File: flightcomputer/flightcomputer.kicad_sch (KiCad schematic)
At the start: 65 parts, among them J1 Conn_Coaxial, J10 Conn_01x03, J11 Conn_01x03, J12 282837-2, J13 282837-2, J2 Conn_Coaxial, J3 Conn_Coaxial, J4 Conn_Coaxial, J5 Conn_01x24, J6 Conn_01x24, J7 Conn_01x01, J8 Conn_01x01, J9 Conn_01x02, M1 Motor_Servo, M2 Motor_Servo, Q1 MMBT3904, Q2 MMBT3904, Q3 SI4925DDY-T1-GE3, U1 MAX-M10S, U2 LIS2MDLTR, U3 BMI088, U4 MS5607-02BA, U5 MIC29302AWD-TR, U6 RFM95W-915S2, U7 Teensy4.1, U8 LD1117S50TR_SOT223

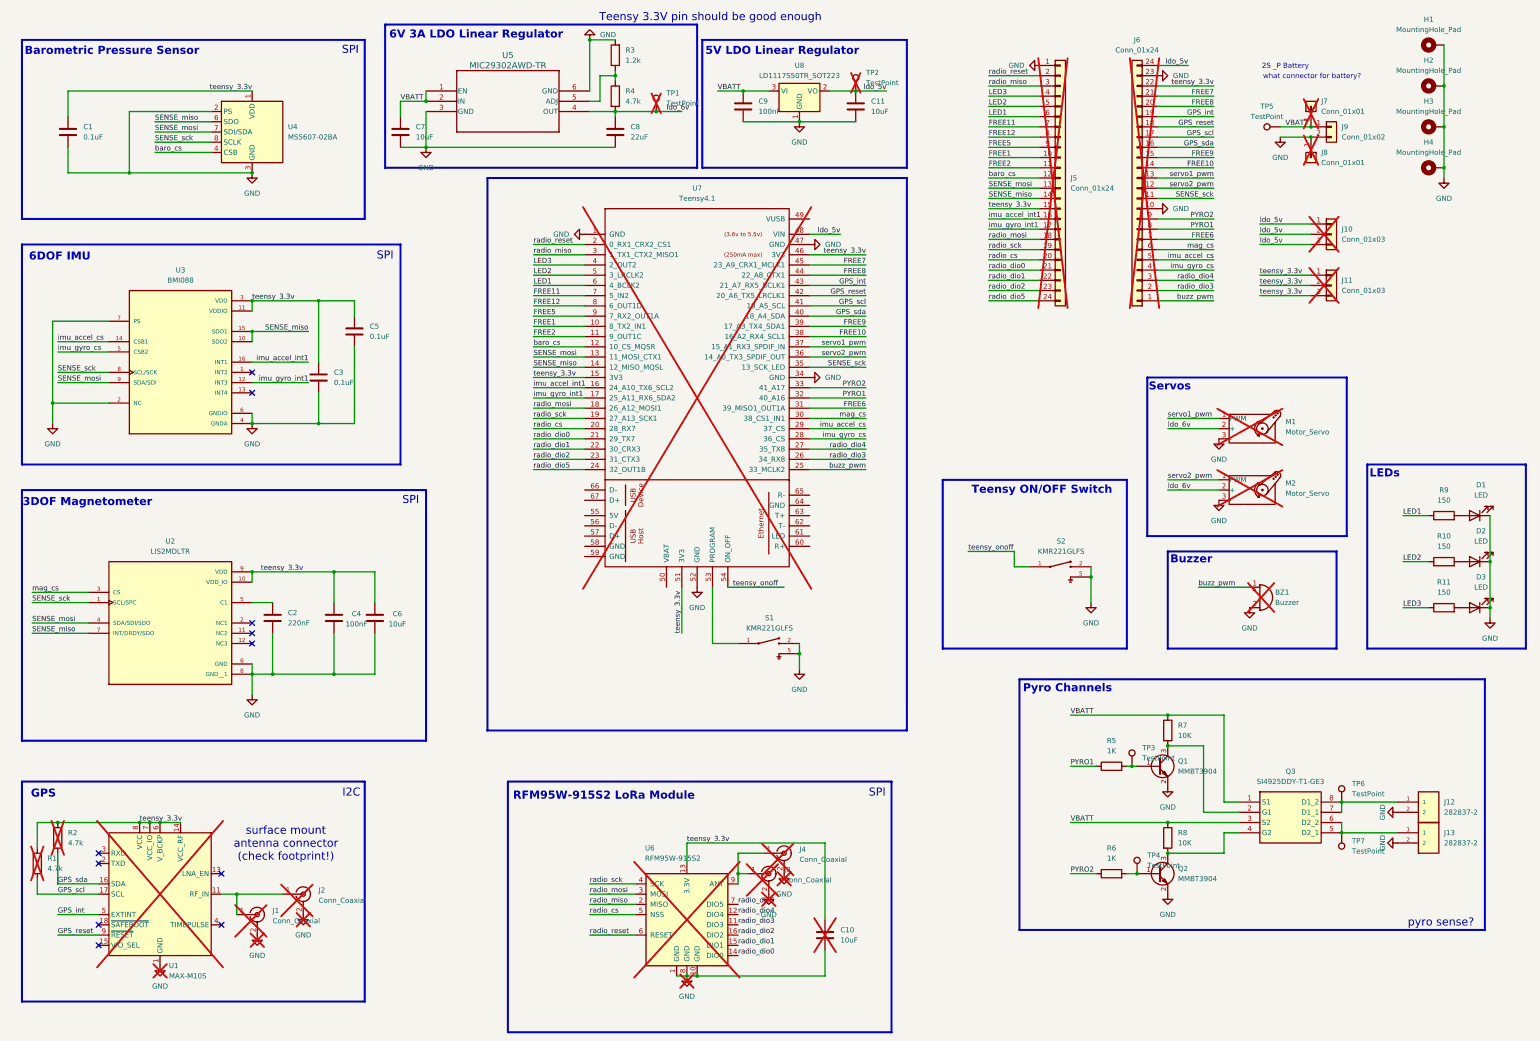
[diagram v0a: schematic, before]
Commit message: all boards
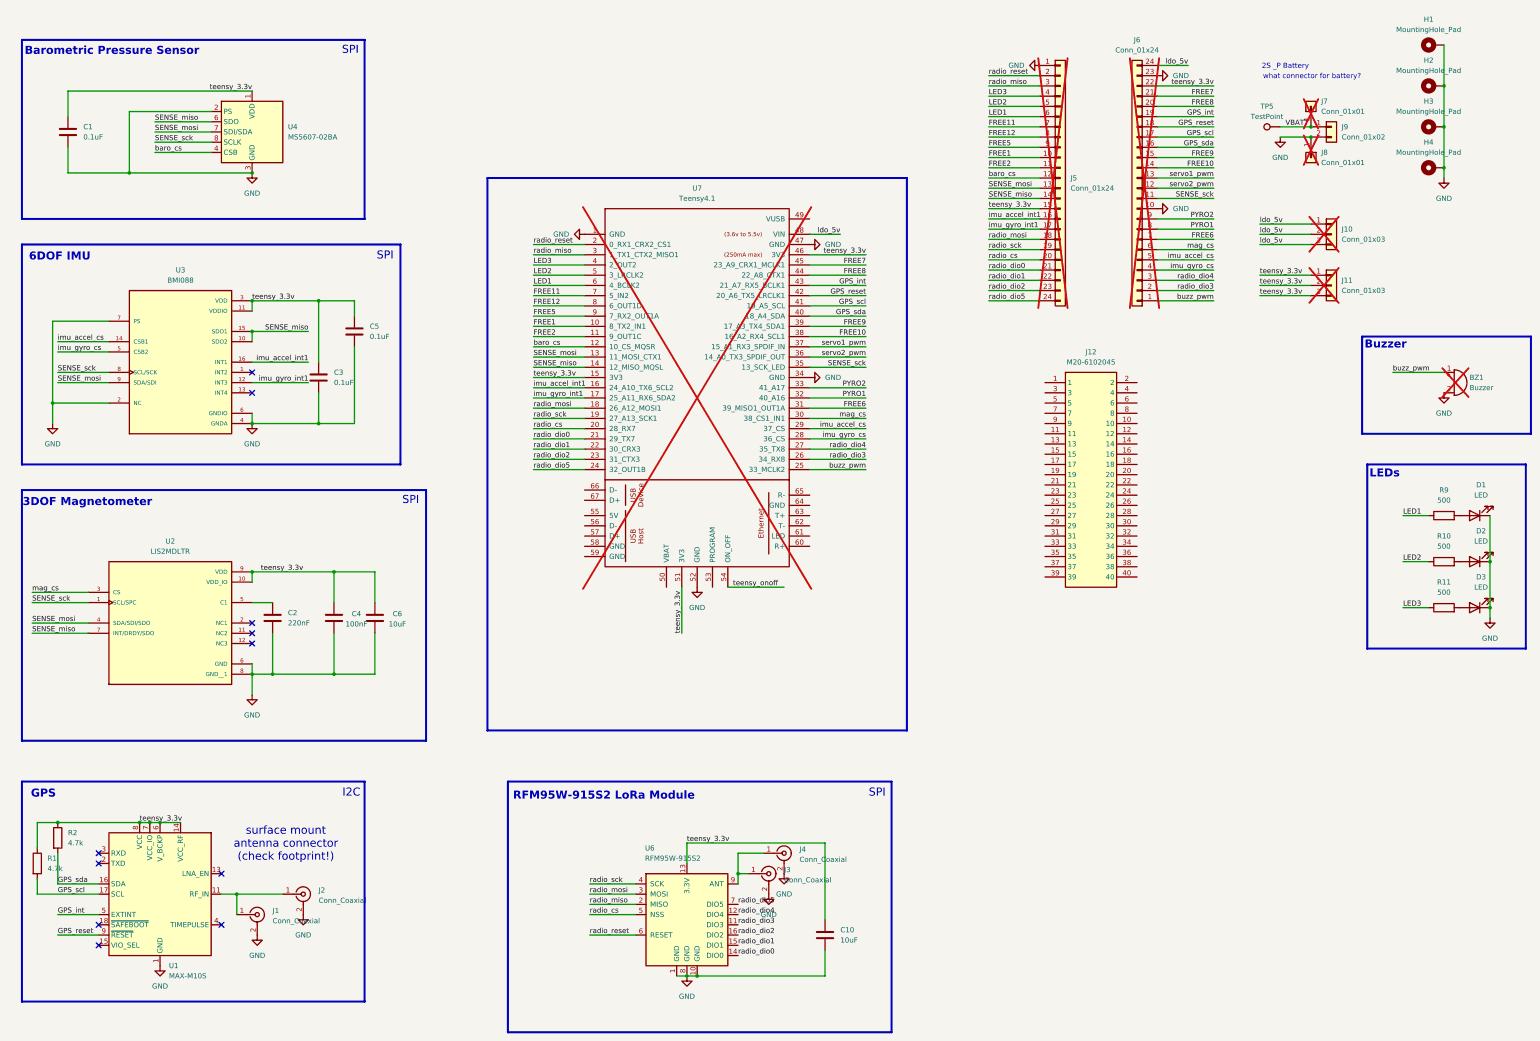
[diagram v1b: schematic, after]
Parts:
- removed C11, C7: 10uF, Capacitor_SMD:C_0603_1608Metric_Pad1.08x0.95mm_HandSolder, symbol Device:C
- removed C8: 22uF, Capacitor_SMD:C_0603_1608Metric_Pad1.08x0.95mm_HandSolder, symbol Device:C
- removed C9: 100nF, Capacitor_SMD:C_0603_1608Metric_Pad1.08x0.95mm_HandSolder, symbol Device:C
- removed J12, J13: 282837-2, HPRfootprints:TE_282837-2, symbol HPRsymbols:282837-2
- removed M1, M2: Motor_Servo, Connector_PinHeader_2.54mm:PinHeader_1x03_P2.54mm_Vertical, symbol Motor:Motor_Servo
- removed Q1, Q2: MMBT3904, Package_TO_SOT_SMD:SOT-23, symbol Transistor_BJT:MMBT3904
- removed Q3: SI4925DDY-T1-GE3, HPRfootprints:SOIC127P600X175-8N, symbol HPRsymbols:SI4925DDY-T1-GE3
- removed R3: 1.2k, Resistor_SMD:R_0603_1608Metric_Pad0.98x0.95mm_HandSolder, symbol Device:R
- removed R4: 4.7k, Resistor_SMD:R_0603_1608Metric_Pad0.98x0.95mm_HandSolder, symbol Device:R
- removed R5, R6: 1K, Resistor_SMD:R_0603_1608Metric_Pad0.98x0.95mm_HandSolder, symbol Device:R
- removed R7, R8: 10K, Resistor_SMD:R_0603_1608Metric_Pad0.98x0.95mm_HandSolder, symbol Device:R
- removed S1, S2: KMR221GLFS, HPRfootprints:SW_KMR221GLFS, symbol HPRsymbols:KMR221GLFS
- removed TP1, TP2: TestPoint, Connector_PinHeader_2.54mm:PinHeader_1x01_P2.54mm_Vertical, symbol Connector:TestPoint
- removed TP3, TP4, TP6, TP7: TestPoint, TestPoint:TestPoint_Pad_1.0x1.0mm, symbol Connector:TestPoint
- removed U5: MIC29302AWD-TR, HPRfootprints:TO-252-5_MCH, symbol HPRsymbols:MIC29302AWD-TR
- removed U8: LD1117S50TR_SOT223, Package_TO_SOT_SMD:SOT-223-3_TabPin2, symbol Regulator_Linear:LD1117S50TR_SOT223
- added J12: M20-6102045, RHDR40W66P254_2X20_5146X500X1105P, symbol HPRsymbols:M20-6102045
- C10, J1, J2, J3, J4, R1, R2, U1, U6: now fitted
- R10, R11, R9: value 150 -> 500
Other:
- note removed: "5V LDO Linear Regulator"
- note removed: "6V 3A LDO Linear Regulator"
- note removed: "Pyro Channels"
- note removed: "Servos"
- note removed: "Teensy 3.3V pin should be good enough"
- note removed: "Teensy ON/OFF Switch"
- note removed: "pyro sense?"
- moved on the sheet: BZ1
